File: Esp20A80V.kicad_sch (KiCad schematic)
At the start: 22 parts, among them J1 dcdc, J2 free, J4 I2C/Uart, Q1 SI2305, SW1 3x button, U1 spi tft with touch (+ sd card), U3 20A 80V dcdc, U4 Wemos S2 Mini

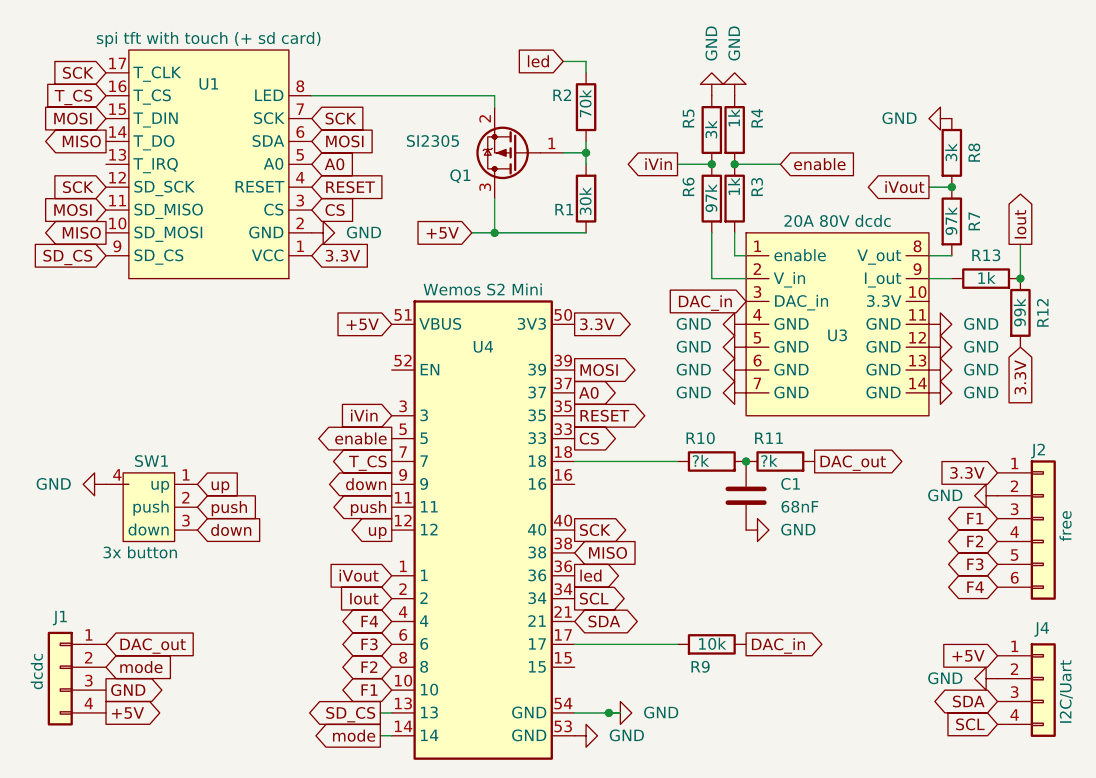
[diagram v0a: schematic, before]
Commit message: update
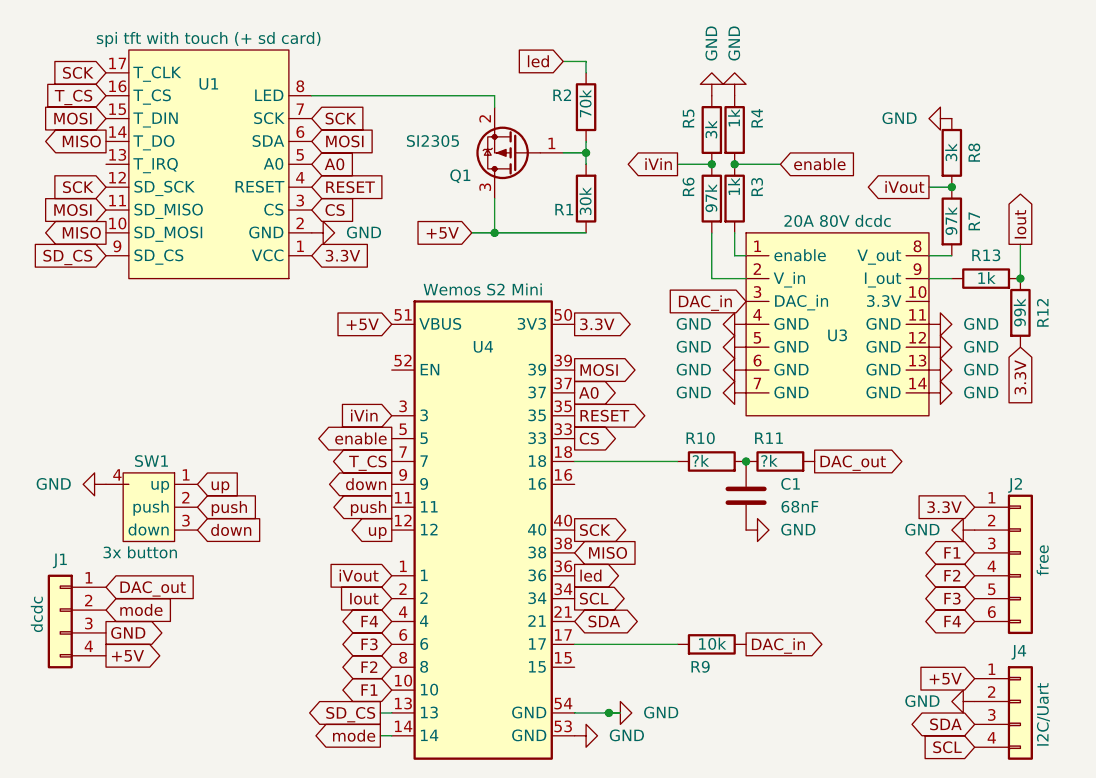
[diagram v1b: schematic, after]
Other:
- moved on the sheet: J1, J2, J4
